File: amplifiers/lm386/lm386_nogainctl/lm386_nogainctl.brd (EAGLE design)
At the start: 51.7 x 40.4 mm, 18 parts, among them IC1 LM386N-4

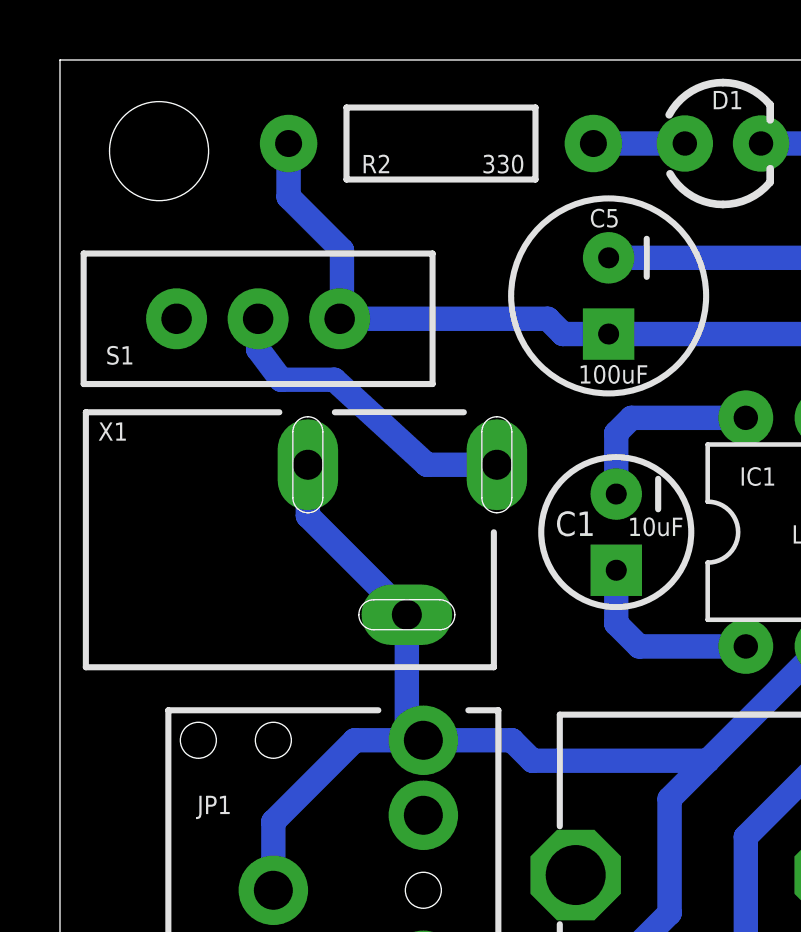
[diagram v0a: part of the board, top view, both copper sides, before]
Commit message: spacing update (just guessing)
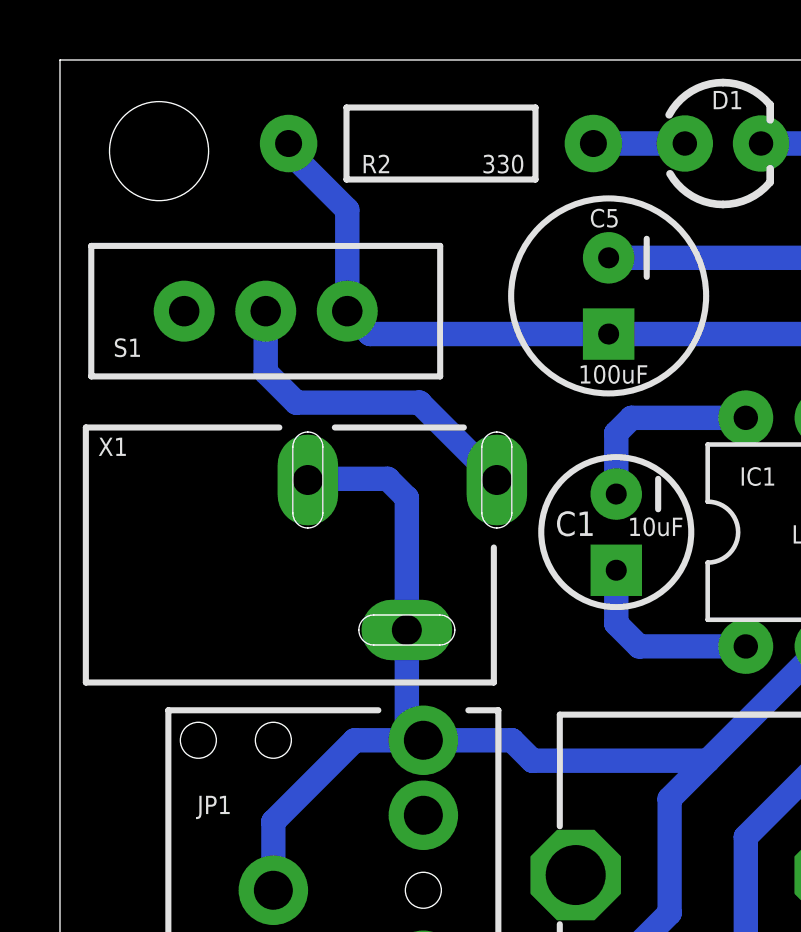
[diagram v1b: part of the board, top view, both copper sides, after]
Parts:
- moved X1 0.51 mm to (0.76, 22.1)
- moved S1 0.36 mm to (6.86, 30.2)
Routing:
- net GND: track 151.9 -> 153.0 mm
- net N$3: track 10.6 -> 11.2 mm
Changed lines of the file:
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@@
 <?xml version="1.0" encoding="utf-8"?>
 <!DOCTYPE eagle SYSTEM "eagle.dtd">
-<eagle version="7.4.0">
+<eagle version="8.7.0">
 <drawing>
 <settings>
 <setting alwaysvectorfont="no"/>
+<setting keepoldvectorfont="yes"/>
 <setting verticaltext="up"/>
 </settings>
@@
 <param name="dpMaxLengthDifference" value="10mm"/>
 <param name="dpGapFactor" value="2.5"/>
-<param name="checkGrid" value="0"/>
 <param name="checkAngle" value="0"/>
 <param name="checkFont" value="1"/>
 <param name="checkRestrict" value="1"/>
+<param name="checkStop" value="0"/>
+<param name="checkValues" value="0"/>
 <param name="useDiameter" value="13"/>
 <param name="maxErrors" value="50"/>
@@
 </element>
 <element name="C5" library="SparkFun-Capacitors" package="CPOL-RADIAL-100UF-25V" value="100uF" x="18.288" y="30.734" smashed="yes" rot="R270">
+<attribute name="NAME" x="17.653" y="33.02" size="0.6096" layer="25" font="vector" ratio="15"/>
 <attribute name="PROD_ID" value="CAP-08439" x="18.288" y="30.734" size="1.778" layer="27" rot="R270" display="off"/>
 <attribute name="VALUE" x="17.272" y="27.813" size="0.6096" layer="21" font="vector" ratio="15"/>
-<attribute name="NAME" x="17.653" y="33.02" size="0.6096" layer="25" font="vector" ratio="15"/>
-</element>
-<element name="S1" library="SparkFun-Electromechanical" package="SWITCH-SPDT_LOCK.007S" value="" x="6.604" y="29.972" smashed="yes" rot="R270">
-<attribute name="NAME" x="1.524" y="28.448" size="0.6096" layer="25" font="vector" ratio="15"/>
-<attribute name="VALUE" x="-2.921" y="33.782" size="1.778" layer="27" ratio="10" rot="R270"/>
+</element>
+<element name="S1" library="SparkFun-Electromechanical" package="SWITCH-SPDT_LOCK.007S" value="" x="6.858" y="30.226" smashed="yes" rot="R270">
+<attribute name="NAME" x="1.778" y="28.702" size="0.6096" layer="25" font="vector" ratio="15"/>
+<attribute name="VALUE" x="-2.667" y="34.036" size="1.778" layer="27" ratio="10" rot="R270"/>
 </element>
 <element name="C4" library="SparkFun-Capacitors" package="CAP-PTH-SMALL2" value="0.1uF" x="30.988" y="11.684" smashed="yes" rot="R270">
@@
 <attribute name="VALUE" x="30.48" y="6.858" size="0.6096" layer="21" font="vector" ratio="15"/>
 </element>
-<element name="X1" library="con-shiua-chyuan" package="SCD-014-A" value="" x="0.762" y="22.606" smashed="yes" rot="R270">
-<attribute name="OC_FARNELL" value="unknown" x="0.762" y="22.606" size="1.778" layer="27" rot="R270" display="off"/>
-<attribute name="MPN" value="" x="0.762" y="22.606" size="1.778" layer="27" rot="R270" display="off"/>
-<attribute name="OC_NEWARK" value="unknown" x="0.762" y="22.606" size="1.778" layer="27" rot="R270" display="off"/>
-<attribute name="MF" value="" x="0.762" y="22.606" size="1.778" layer="27" rot="R270" display="off"/>
-<attribute name="NAME" x="1.27" y="25.908" size="0.6096" layer="25" font="vector" ratio="15"/>
-<attribute name="VALUE" x="0.762" y="16.256" size="1.778" layer="27"/>
+<element name="X1" library="con-shiua-chyuan" package="SCD-014-A" value="" x="0.762" y="22.098" smashed="yes" rot="R270">
+<attribute name="MF" value="" x="0.762" y="22.098" size="1.778" layer="27" rot="R270" display="off"/>
+<attribute name="MPN" value="" x="0.762" y="22.098" size="1.778" layer="27" rot="R270" display="off"/>
+<attribute name="NAME" x="1.27" y="25.4" size="0.6096" layer="25" font="vector" ratio="15"/>
+<attribute name="OC_FARNELL" value="unknown" x="0.762" y="22.098" size="1.778" layer="27" rot="R270" display="off"/>
+<attribute name="OC_NEWARK" value="unknown" x="0.762" y="22.098" size="1.778" layer="27" rot="R270" display="off"/>
+<attribute name="VALUE" x="0.762" y="15.748" size="1.778" layer="27"/>
 </element>
 <element name="U$1" library="SparkFun-Electromechanical" package="STAND-OFF" value="" x="3.302" y="35.56"/>
@@
 <wire x1="23.368" y1="35.814" x2="24.892" y2="35.814" width="0.8128" layer="16"/>
 <wire x1="24.892" y1="35.814" x2="28.702" y2="32.004" width="0.8128" layer="16"/>
-<wire x1="8.262" y1="25.106" x2="8.262" y2="23.406" width="0.8128" layer="16"/>
-<wire x1="8.262" y1="23.406" x2="11.562" y2="20.106" width="0.8128" layer="16"/>
-<wire x1="11.562" y1="20.106" x2="11.562" y2="16.472" width="0.8128" layer="16"/>
-<wire x1="11.562" y1="16.472" x2="12.112" y2="15.922" width="0.8128" layer="16"/>
 <wire x1="12.112" y1="15.922" x2="15.066" y2="15.922" width="0.8128" layer="16"/>
 <wire x1="15.066" y1="15.922" x2="15.748" y2="15.24" width="0.8128" layer="16"/>
@@
 <wire x1="30.48" y1="20.32" x2="33.02" y2="20.32" width="0.8128" layer="16"/>
 <wire x1="33.02" y1="20.32" x2="35.56" y2="22.86" width="0.8128" layer="16"/>
+<wire x1="12.112" y1="15.922" x2="11.562" y2="16.472" width="0.8128" layer="16"/>
+<wire x1="11.562" y1="16.472" x2="11.562" y2="19.598" width="0.8128" layer="16"/>
+<wire x1="11.562" y1="19.598" x2="11.562" y2="23.998" width="0.8128" layer="16"/>
+<wire x1="11.562" y1="23.998" x2="10.922" y2="24.638" width="0.8128" layer="16"/>
+<wire x1="10.922" y1="24.638" x2="8.302" y2="24.638" width="0.8128" layer="16"/>
+<wire x1="8.302" y1="24.638" x2="8.262" y2="24.598" width="0.8128" layer="16"/>
 </signal>
 <signal name="N$4">
@@
 <wire x1="26.416" y1="29.464" x2="27.94" y2="27.94" width="0.8128" layer="16"/>
 <wire x1="27.94" y1="27.94" x2="27.94" y2="26.67" width="0.8128" layer="16"/>
-<wire x1="9.398" y1="29.972" x2="16.256" y2="29.972" width="0.8128" layer="16"/>
-<wire x1="16.256" y1="29.972" x2="16.764" y2="29.464" width="0.8128" layer="16"/>
-<wire x1="16.764" y1="29.464" x2="18.288" y2="29.464" width="0.8128" layer="16"/>
 <wire x1="18.288" y1="29.464" x2="26.416" y2="29.464" width="0.8128" layer="16"/>
 <contactref element="R2" pad="P$2"/>
-<wire x1="9.3218" y1="29.972" x2="9.398" y2="29.972" width="0.8128" layer="16"/>
-<wire x1="9.398" y1="29.972" x2="9.398" y2="32.258" width="0.8128" layer="16"/>
-<wire x1="9.398" y1="32.258" x2="7.62" y2="34.036" width="0.8128" layer="16"/>
-<wire x1="7.62" y1="34.036" x2="7.62" y2="35.814" width="0.8128" layer="16"/>
+<wire x1="9.5758" y1="30.226" x2="9.5758" y2="33.6042" width="0.8128" layer="16"/>
+<wire x1="7.62" y1="35.56" x2="7.62" y2="35.814" width="0.8128" layer="16"/>
+<wire x1="9.5758" y1="33.6042" x2="7.62" y2="35.56" width="0.8128" layer="16"/>
+<wire x1="9.5758" y1="30.226" x2="10.3378" y2="29.464" width="0.8128" layer="16"/>
+<wire x1="10.3378" y1="29.464" x2="18.288" y2="29.464" width="0.8128" layer="16"/>
 </signal>
 <signal name="N$5">
@@
 <contactref element="S1" pad="2"/>
 <contactref element="X1" pad="1"/>
-<wire x1="14.562" y1="25.106" x2="12.232" y2="25.106" width="0.8128" layer="16"/>
-<wire x1="12.232" y1="25.106" x2="9.144" y2="27.94" width="0.8128" layer="16"/>
-<wire x1="9.144" y1="27.94" x2="7.366" y2="27.94" width="0.8128" layer="16"/>
-<wire x1="7.366" y1="27.94" x2="6.604" y2="28.956" width="0.8128" layer="16"/>
-<wire x1="6.604" y1="28.956" x2="6.604" y2="29.972" width="0.8128" layer="16"/>
+<wire x1="14.562" y1="24.598" x2="11.982" y2="27.178" width="0.8128" layer="16"/>
+<wire x1="7.874" y1="27.178" x2="6.858" y2="28.194" width="0.8128" layer="16"/>
+<wire x1="11.982" y1="27.178" x2="7.874" y2="27.178" width="0.8128" layer="16"/>
+<wire x1="6.858" y1="28.194" x2="6.858" y2="30.226" width="0.8128" layer="16"/>
 </signal>
 <signal name="N$10">
